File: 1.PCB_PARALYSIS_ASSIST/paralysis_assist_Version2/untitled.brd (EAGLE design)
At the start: 127 x 100 mm, 33 parts, among them IC2 7805TV, SW1 1825910-2, SW2 1825910-2, U1 ZC563900

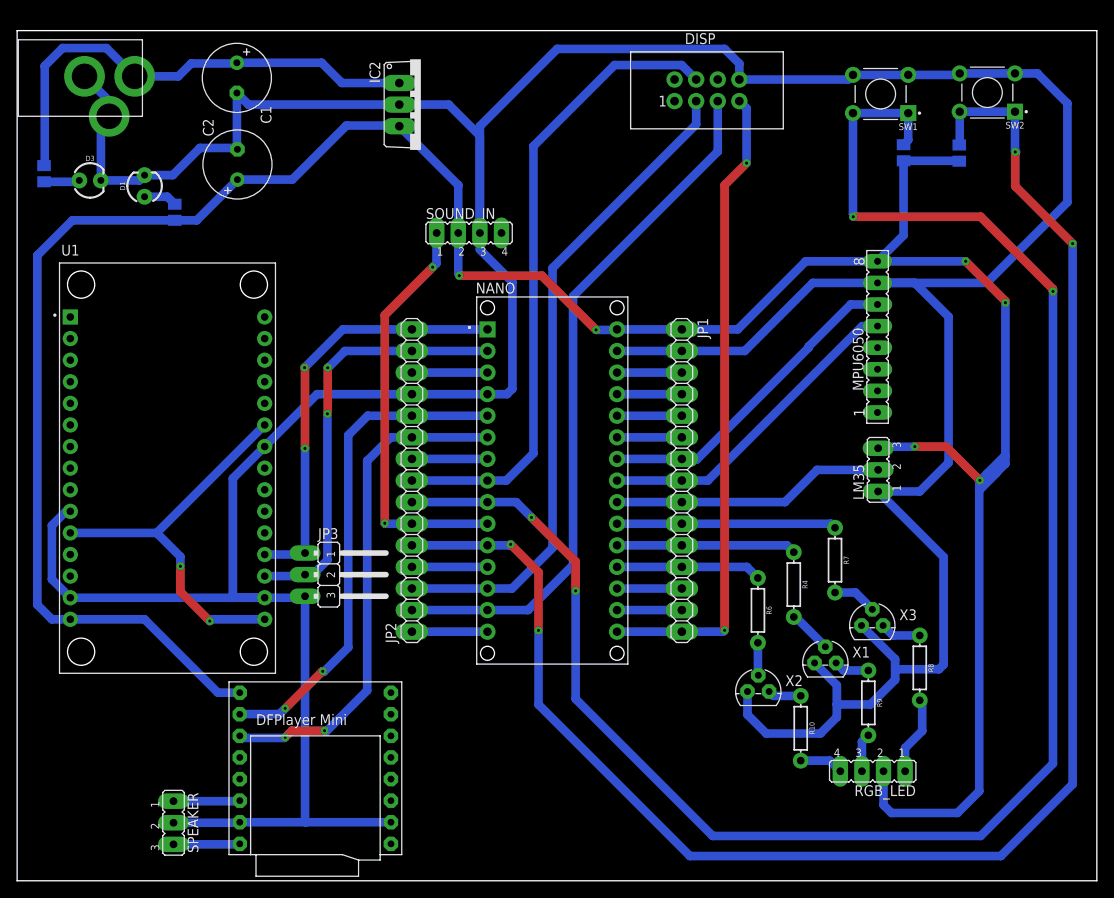
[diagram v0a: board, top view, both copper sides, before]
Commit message: corrections to the pcb
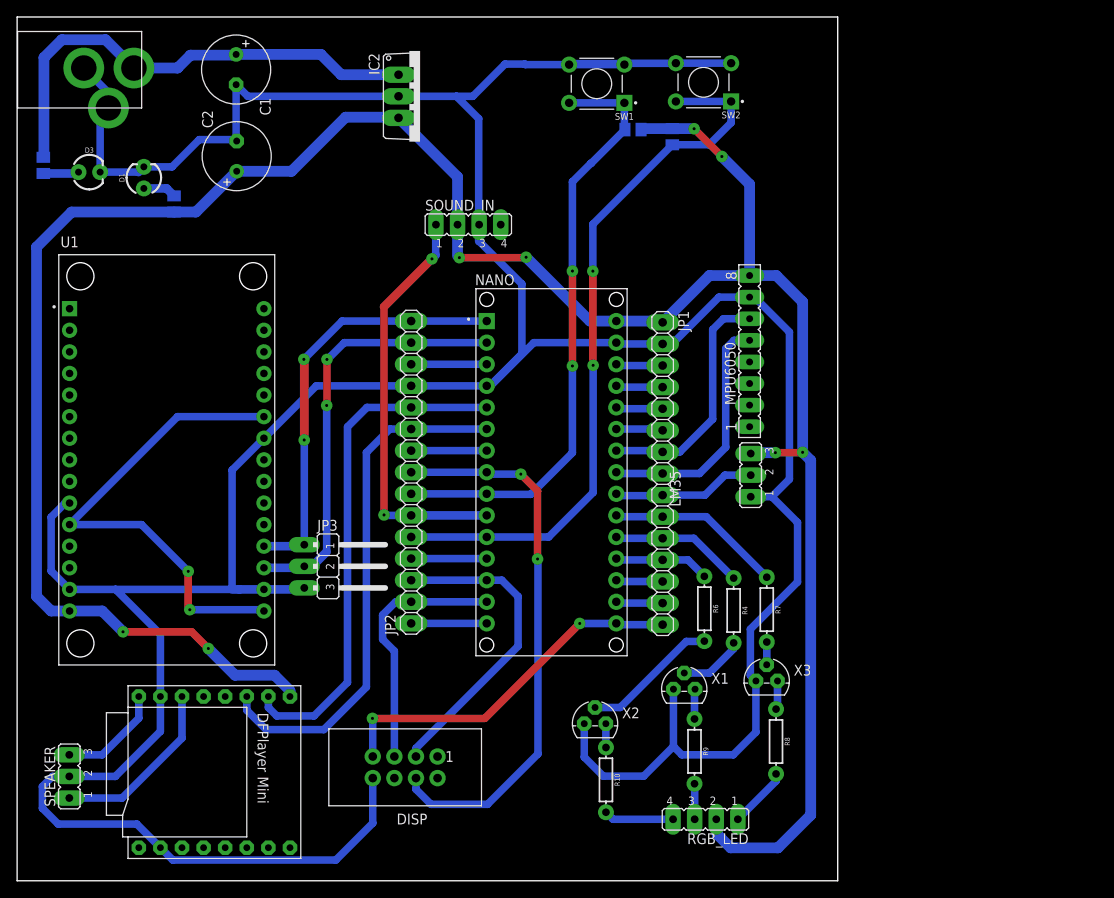
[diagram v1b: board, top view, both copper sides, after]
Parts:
- moved DISP 87.2 mm to (45.6, 13.3), turned to 180 degrees
- moved R2 33.8 mm to (77.1, 87.5), turned to 270 degrees
- moved SW1 33.4 mm to (71.4, 91.5)
- moved SW2 33.4 mm to (84.0, 91.7)
- moved R3 31.9 mm to (72.4, 88.4), turned to 0 degrees
- moved R10 23.7 mm to (69.3, 11.9)
- moved R9 21.2 mm to (79.7, 15.2)
- moved RGB_LED 20.5 mm to (81.0, 7.24)
- moved X2 19.6 mm to (68.0, 18.5)
- moved R8 19.0 mm to (89.3, 16.4)
- moved X1 16.9 mm to (78.5, 22.5)
- moved MPU6050 15.1 mm to (86.2, 62.3)
- moved LM35 15.0 mm to (86.3, 47.7)
- moved X3 14.0 mm to (88.2, 23.5)
- moved SPEAKER 13.4 mm to (6.14, 12.3), turned to 90 degrees
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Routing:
- net OK: track 210.2 -> 71.3 mm, vias 4 -> 2
- net BACK: track 198.1 -> 85.4 mm, vias 4 -> 2
- net GND: track 514.7 -> 443.9 mm
- net MOSI: track 82.8 -> 30.1 mm
- net CS_DISP: track 78.1 -> 37.2 mm
- net SCK: track 76.4 -> 43.3 mm
- net 5V: track 326.4 -> 300.1 mm, vias 6 -> 8
- net TEMP: track 32.3 -> 16.9 mm
- net SPK_1: track 7.82 -> 21.1 mm
- net BASE_BLUE: track 3.85 -> 16.1 mm
- net 3V3: track 47.6 -> 57.8 mm
- net RST: track 75.6 -> 65.6 mm, vias 0 -> 2
- net SCL: track 38.3 -> 28.4 mm
- net SDA: track 38.2 -> 29.0 mm
- net A0: track 17.1 -> 11.2 mm
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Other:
- board size 127 x 100 mm -> 96.5 x 101.6 mm
